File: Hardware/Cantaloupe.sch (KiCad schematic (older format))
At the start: 141 parts, among them J1 BAT_CON, J2 OLED, J3 Interconnect, J4 ICSP, J5 BAT_CON_TOG, J6 OLED, J7 Interconnect_R, J8 ICSP_R, J9 BAT_CON_R, SW1 MX, SW10 MX, SW11 MX, SW12 MX, SW13 MX, SW14 MX, SW15 MX, SW16 MX, SW17 MX, SW18 MX, SW19 MX, SW2 MX, SW20 MX, SW21 MX, SW22 MX, SW23 MX, SW24 MX, SW25 MX, SW26 MX, SW27 MX, SW28 MX, SW29 MX, SW3 MX, SW30 MX, SW31 Reset, SW32 5_Way, SW33 BAT_TOG, SW34 Encoder, SW35 MX, SW36 MX, SW37 MX, SW38 MX, SW39 MX, SW4 MX, SW40 MX, SW41 MX, SW42 MX, SW43 MX, SW44 MX, SW45 MX, SW46 MX, SW47 MX, SW48 MX, SW49 MX, SW5 MX, SW50 MX, SW51 MX, SW52 MX, SW53 MX, SW54 MX, SW55 MX, SW56 MX, SW57 MX, SW58 MX, SW59 MX, SW6 MX, SW60 MX, SW61 MX, SW62 MX, SW63 MX, SW64 MX, SW65 Reset, SW66 5_Way_R, SW67 Encoder_R, SW68 BAT_TOG_R, SW7 MX, SW8 MX, SW9 MX, U1 ProMicro, U2 ProMicro

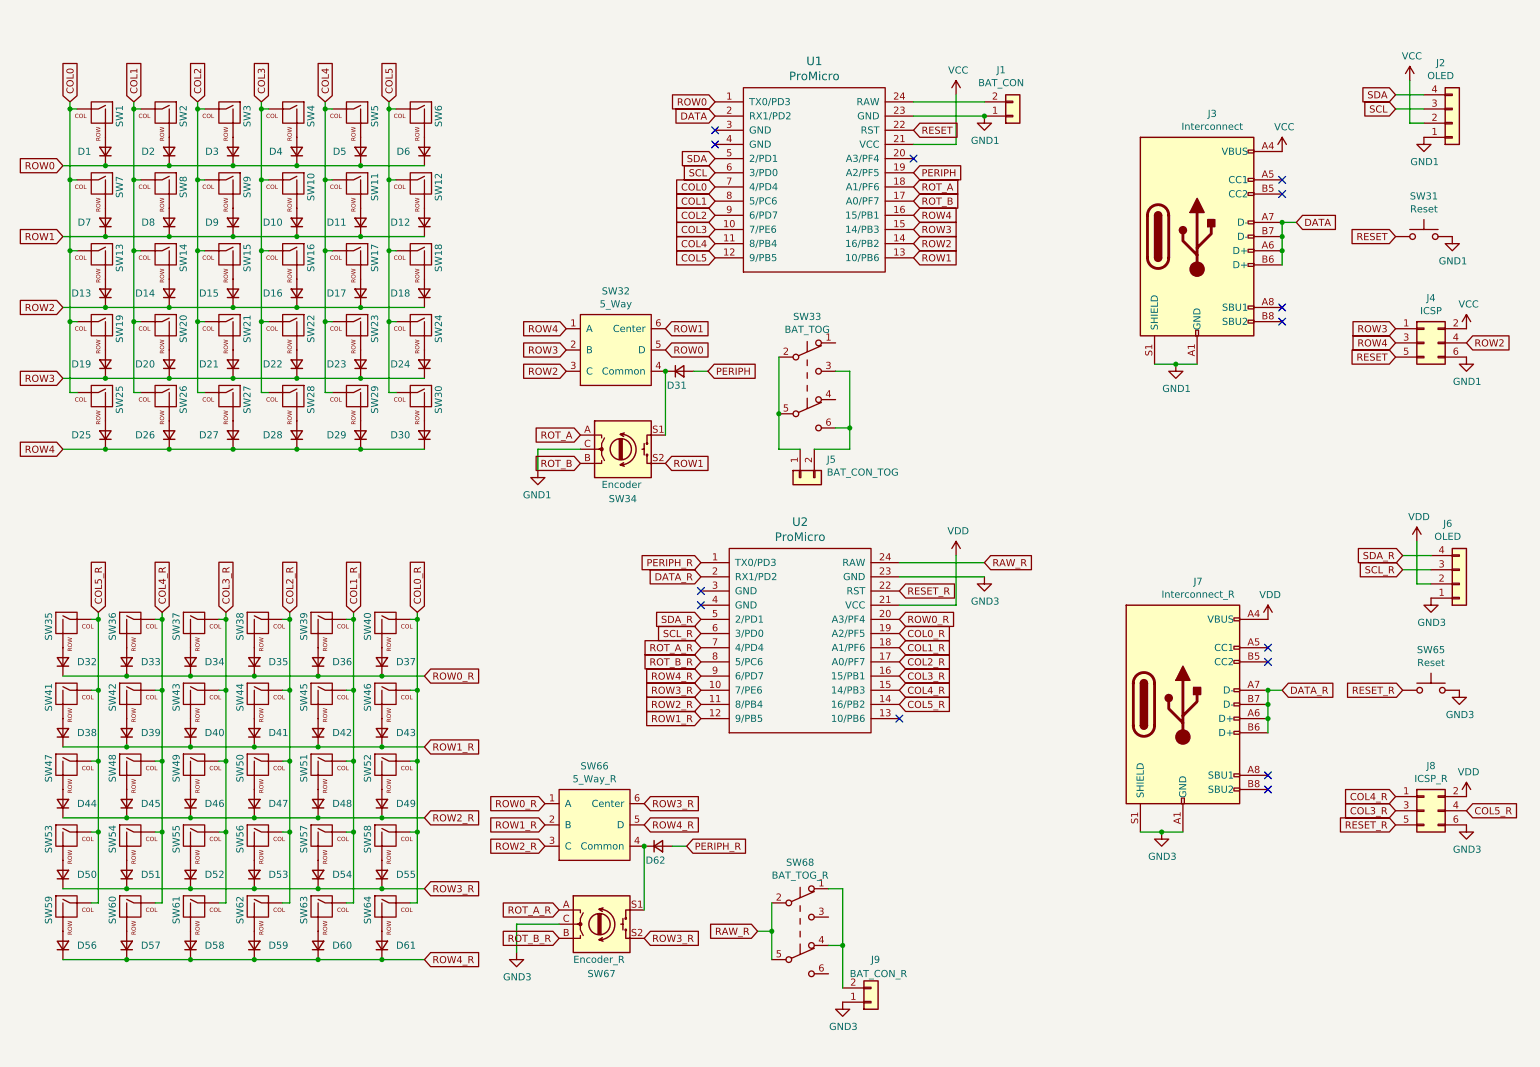
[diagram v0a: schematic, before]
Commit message: Updated to V1.2
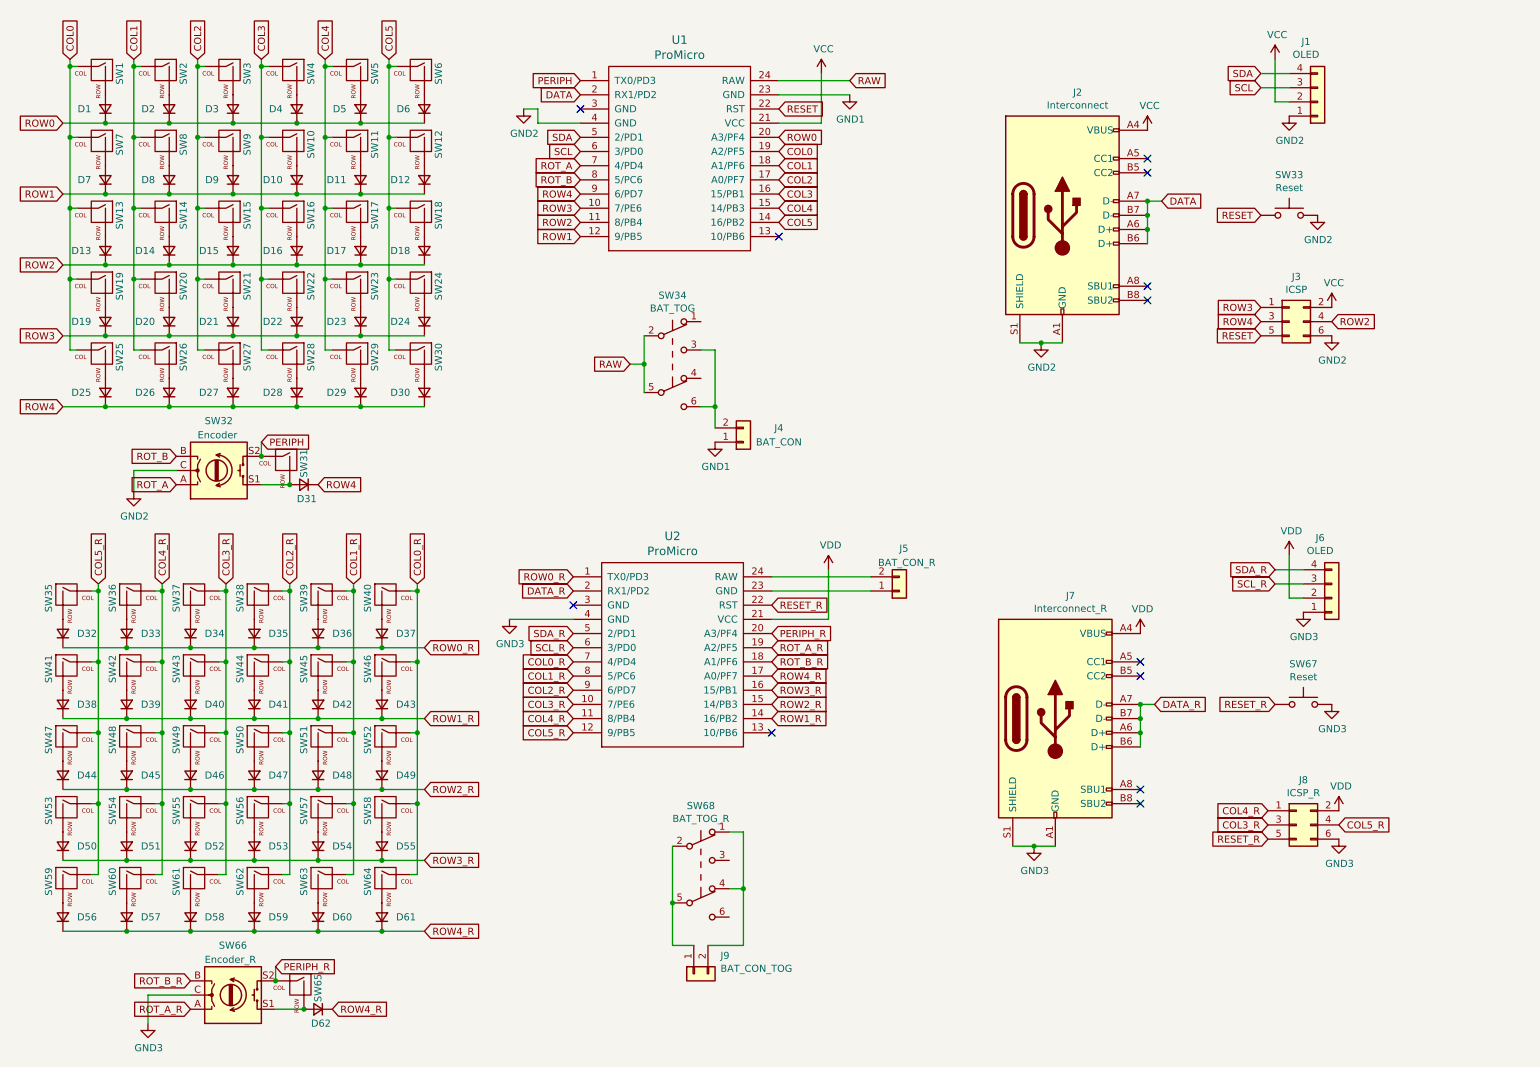
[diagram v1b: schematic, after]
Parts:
- removed SW32: 5_Way, Cantaloupe:Switch_5-way-tactile, symbol Cantaloupe:Switch_5-Way-Tactile
- removed SW66: 5_Way_R, Cantaloupe:Switch_5-way-tactile, symbol Cantaloupe:Switch_5-Way-Tactile
- added SW31, SW65: MX, Cantaloupe:HYBRID-MX_ALPS_SMK-1U, symbol Cantaloupe:MX-NoLED
- D1, D10, D11, D12, D13, D14, D15, D16, D17, D18, D19, D2, D20, D21, D22, D23, D24, D25, D26, D27, D28, D29, D3, D30, D31, D32, D33, D34, D35, D36, D37, D38, D39, D4, D40, D41, D42, D43, D44, D45, D46, D47, D48, D49, D5, D50, D51, D52, D53, D54, D55, D56, D57, D58, D59, D6, D60, D61, D62, D7, D8, D9: footprint Diode_SMD:D_SOD-123 -> Cantaloupe:D_Hybrid_SOD123_DO35
- SW1, SW10, SW11, SW12, SW13, SW14, SW15, SW16, SW17, SW18, SW19, SW2, SW20, SW21, SW22, SW23, SW24, SW25, SW26, SW27, SW28, SW29, SW3, SW30, SW35, SW36, SW37, SW38, SW39, SW4, SW40, SW41, SW42, SW43, SW44, SW45, SW46, SW47, SW48, SW49, SW5, SW50, SW51, SW52, SW53, SW54, SW55, SW56, SW57, SW58, SW59, SW6, SW60, SW61, SW62, SW63, SW64, SW7, SW8, SW9: footprint Cantaloupe:MX-1U-Hotswap -> Cantaloupe:HYBRID-MX_ALPS_SMK-1U
- renumbered J2 to J1, J3 to J2, J4 to J3, J1 to J4, J9 to J5, J5 to J9, SW34 to SW32, SW31 to SW33, SW33 to SW34, SW67 to SW66, SW65 to SW67
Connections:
- net COL0: now also U1.19 (A2/PF5); no longer U1.7 (4/PD4)
- net COL0_R: now also U2.7 (4/PD4); no longer U2.19 (A2/PF5)
- net COL1: now also U1.18 (A1/PF6); no longer U1.8 (5/PC6)
- net COL1_R: now also U2.8 (5/PC6); no longer U2.18 (A1/PF6)
- net COL2: now also U1.17 (A0/PF7); no longer U1.9 (6/PD7)
- net COL2_R: now also U2.9 (6/PD7); no longer U2.17 (A0/PF7)
- net COL3: now also U1.16 (15/PB1); no longer U1.10 (7/PE6)
- net COL3_R: now also U2.10 (7/PE6); no longer U2.16 (15/PB1)
- net COL4: now also U1.15 (14/PB3); no longer U1.11 (8/PB4)
- net COL4_R: now also U2.11 (8/PB4); no longer U2.15 (14/PB3)
- net COL5: now also U1.14 (16/PB2); no longer U1.12 (9/PB5)
- net COL5_R: now also U2.12 (9/PB5); no longer U2.14 (16/PB2)
- net GND1: no longer J1.1 (Pin_1), J2.A1 (GND), J2.A12 (GND), J2.B1 (GND), J2.B12 (GND), J2.S1 (SHIELD), J3.6 (Pin_6), SW32.C, SW33.2
- net GND3: now also U2.4 (GND); no longer J5.1 (Pin_1), U2.23 (GND)
- net PERIPH: now also SW32.S2, U1.1 (TX0/PD3), SW31.1 (COL); no longer D31.2 (A), U1.19 (A2/PF5)
- net PERIPH_R: now also SW66.S2, U2.20 (A3/PF4), SW65.1 (COL); no longer D62.2 (A), U2.1 (TX0/PD3)
- net ROT_A: now also U1.7 (4/PD4); no longer U1.18 (A1/PF6)
- net ROT_A_R: now also U2.19 (A2/PF5); no longer U2.7 (4/PD4)
- net ROT_B: now also U1.8 (5/PC6); no longer U1.17 (A0/PF7)
- net ROT_B_R: now also U2.18 (A1/PF6); no longer U2.8 (5/PC6)
- net ROW0: now also U1.20 (A3/PF4); no longer U1.1 (TX0/PD3)
- net ROW0_R: now also U2.1 (TX0/PD3); no longer U2.20 (A3/PF4)
- net ROW1: now also U1.12 (9/PB5); no longer SW32.S2, U1.13 (10/PB6)
- net ROW1_R: now also U2.14 (16/PB2); no longer U2.12 (9/PB5)
- net ROW2: now also U1.11 (8/PB4); no longer U1.14 (16/PB2)
- net ROW2_R: now also U2.15 (14/PB3); no longer U2.11 (8/PB4)
- net ROW3: now also U1.10 (7/PE6); no longer U1.15 (14/PB3)
- net ROW3_R: now also U2.16 (15/PB1); no longer SW66.S2, U2.10 (7/PE6)
- net ROW4: now also D31.1 (K), U1.9 (6/PD7); no longer U1.16 (15/PB1)
- net ROW4_R: now also D62.1 (K), U2.17 (A0/PF7); no longer U2.9 (6/PD7)
- net at J4.2 (Pin_2): now also SW34.3 (C), SW34.6 (C); no longer U1.24 (RAW)
- net GND2: now reaches U1.4 (GND)
- net GND2: now also J1.1 (Pin_1), J2.A1 (GND), J2.A12 (GND), J2.B1 (GND), J2.B12 (GND), J2.S1 (SHIELD), J3.6 (Pin_6), SW32.C, SW33.2
- net at SW32.S1: now also D31.2 (A), SW31.2 (ROW); no longer D31.1 (K)
- net RAW: now reaches SW34.2 (B), SW34.5 (B)
- net RAW: now also U1.24 (RAW); no longer J9.1 (Pin_1)
- net at SW68.1 (A), SW68.4 (A): now also J9.2 (Pin_2); no longer J5.2 (Pin_2)
- net at SW66.S1: now also D62.2 (A), SW65.2 (ROW); no longer D62.1 (K)
- net RAW_R: no longer names the net of SW68.2 (B), SW68.5 (B)
- net RAW_R: now also J9.1 (Pin_1); no longer U2.24 (RAW)
- new net: J5.1 (Pin_1), U2.23 (GND)
- new net: J5.2 (Pin_2), U2.24 (RAW)
- no-connect marks 14 -> 12
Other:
- moved on the sheet: D1, D10, D11, D12, D13, D14, D15, D16, D17, D18, D19, D2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
